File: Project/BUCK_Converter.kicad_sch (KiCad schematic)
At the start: 17 parts, among them J601 Screw_Terminal_01x04, U601 MAX15062AATA+T

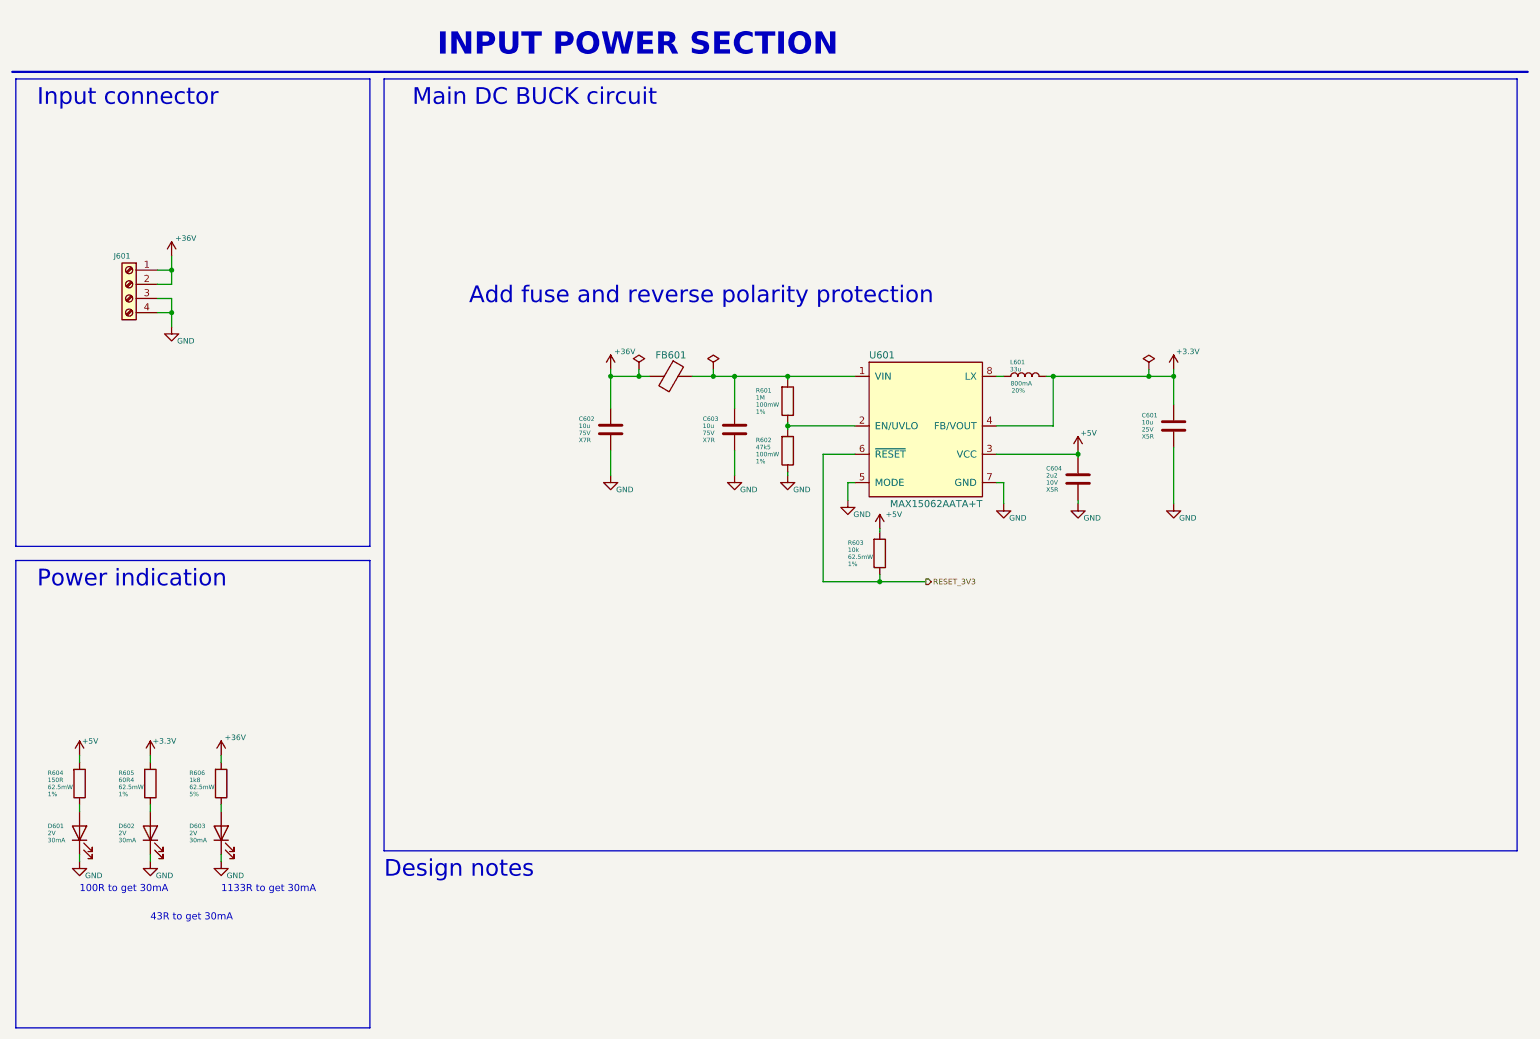
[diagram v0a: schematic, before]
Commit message: Cleanup ED A1 version
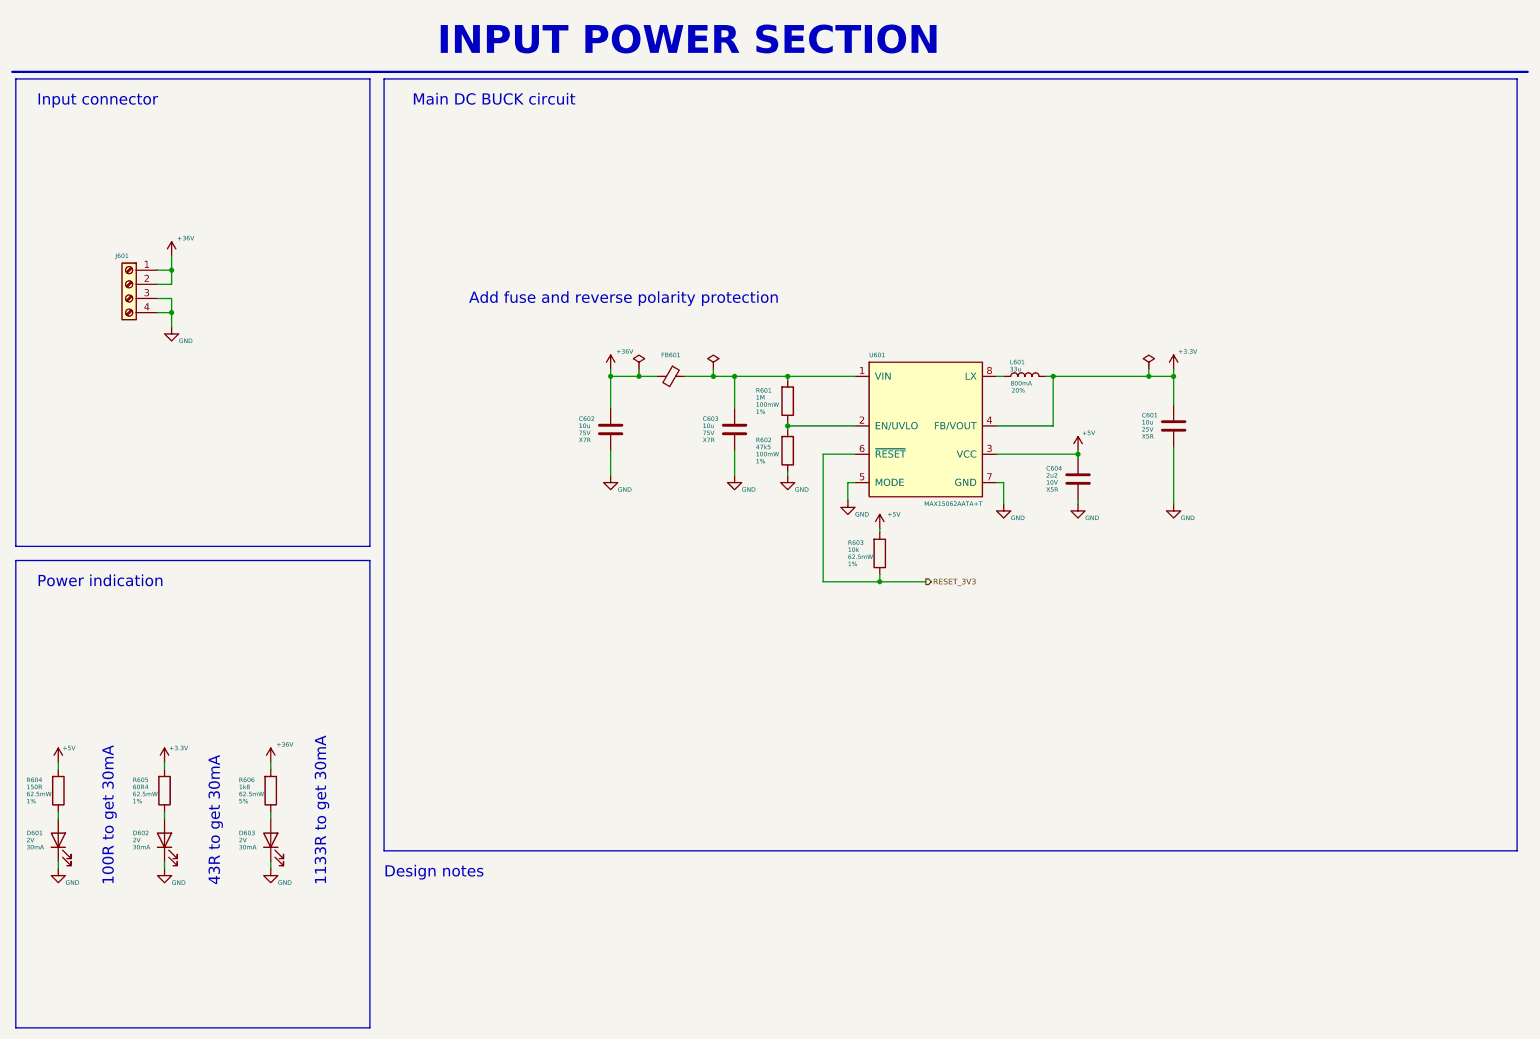
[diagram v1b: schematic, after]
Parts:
- FB601: symbol Device:Ferrite_Bead -> Device:FerriteBead_Small
- U601: symbol eval_board_tmc6200-ta-rescue:MAX15062BATA+T-eval_board_tmc6200-ta -> QP_LIBRARY:MAX15062BATA+T
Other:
- moved on the sheet: D601, D602, D603, R604, R605, R606
